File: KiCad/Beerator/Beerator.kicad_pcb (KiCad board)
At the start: 4 copper layers, 112 x 52 mm, 55 parts, among them SW1 SW_DPDT_x2, Y401 16MHz

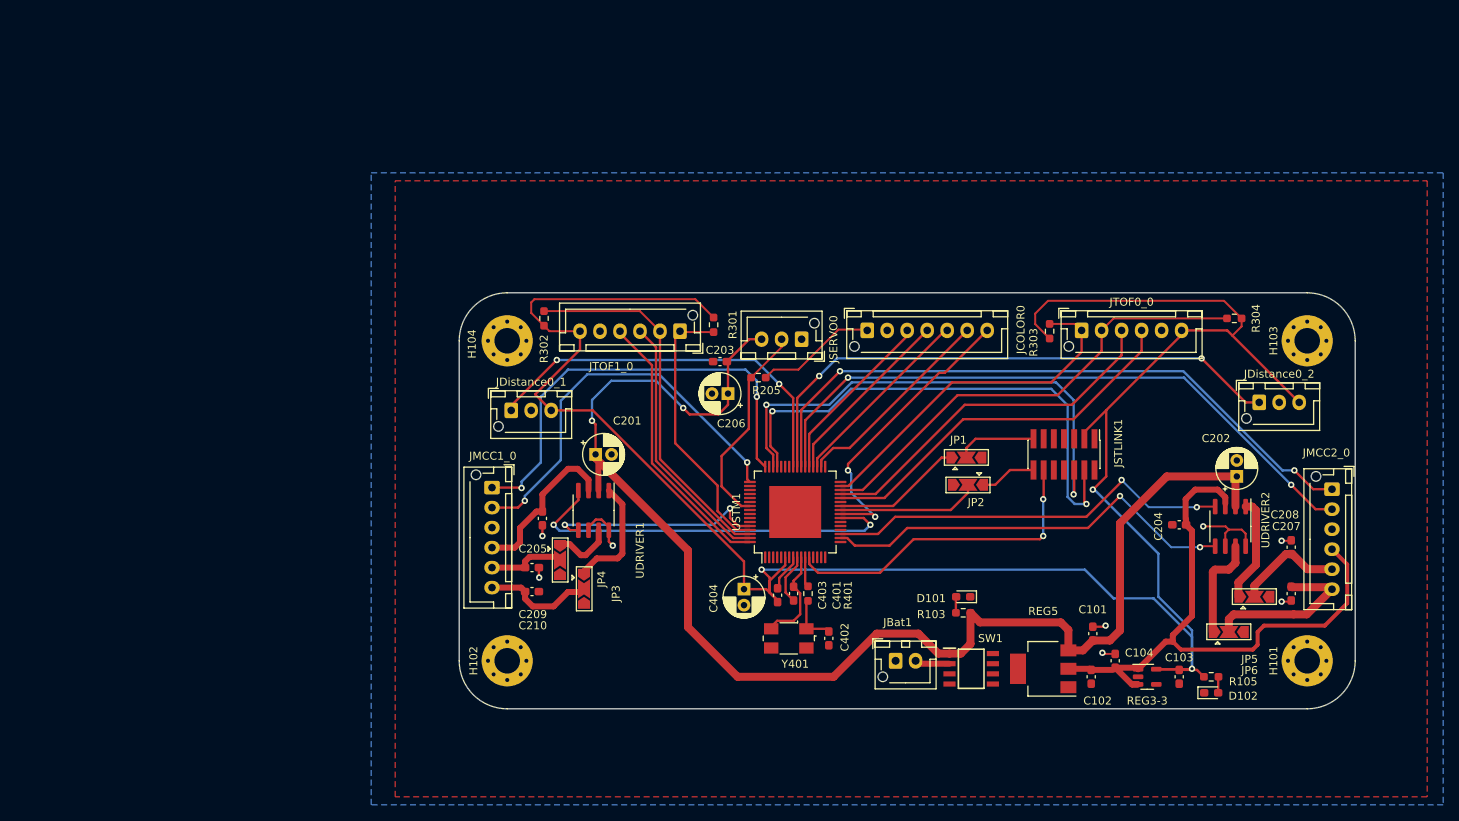
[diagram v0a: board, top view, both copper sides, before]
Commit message: pcb_v2
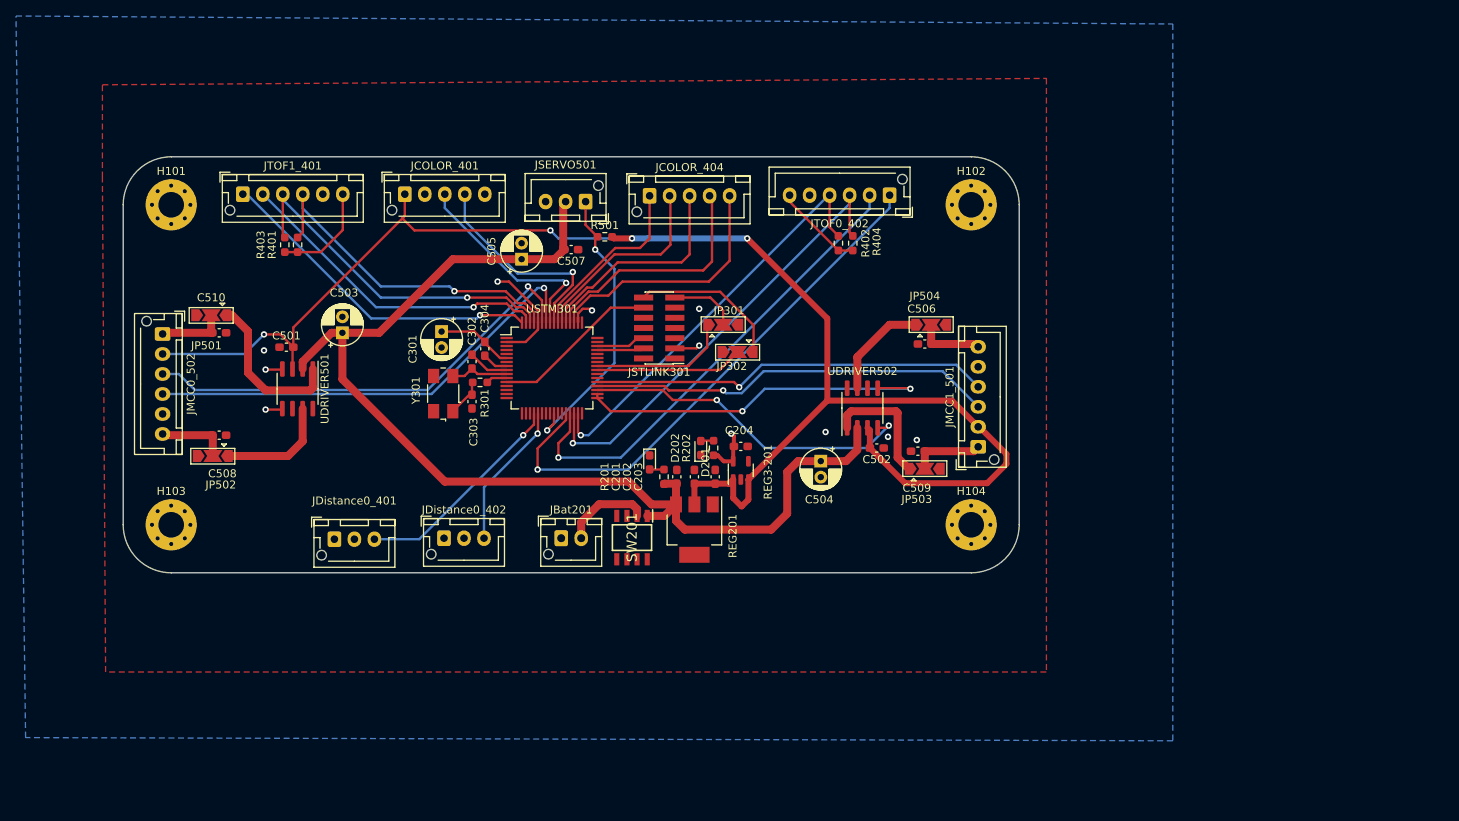
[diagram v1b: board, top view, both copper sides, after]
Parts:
- removed C101: 10uF, Capacitor_SMD:C_0603_1608Metric_Pad1.08x0.95mm_HandSolder
- removed C102: 22uF, Capacitor_SMD:C_0603_1608Metric_Pad1.08x0.95mm_HandSolder
- removed C103, C104: 1uF, Capacitor_SMD:C_0603_1608Metric_Pad1.08x0.95mm_HandSolder
- removed C205: 1µF, Capacitor_SMD:C_0603_1608Metric_Pad1.08x0.95mm_HandSolder
- removed C206: 100uF, Capacitor_THT:CP_Radial_D5.0mm_P2.00mm
- removed C207, C208, C209, C210: 0.1uF, Capacitor_SMD:C_0603_1608Metric_Pad1.08x0.95mm_HandSolder
- removed C401, C402: 15p, Capacitor_SMD:C_0603_1608Metric_Pad1.08x0.95mm_HandSolder
- removed C403: 100n, Capacitor_SMD:C_0603_1608Metric_Pad1.08x0.95mm_HandSolder
- removed C404: 4,7u, Capacitor_THT:CP_Radial_D5.0mm_P2.00mm
- removed D101, D102: LED_Small, LED_SMD:LED_0603_1608Metric_Pad1.05x0.95mm_HandSolder
- removed JBat1: Conn_01x02_Female, Connector_JST:JST_XH_B2B-XH-AM_1x02_P2.50mm_Vertical
- removed JCOLOR0: Conn_01x07_Female, Connector_JST:JST_XH_B7B-XH-AM_1x07_P2.50mm_Vertical
- removed JDistance0_1, JDistance0_2, JSERVO0: Conn_01x03_Female, Connector_JST:JST_XH_B3B-XH-AM_1x03_P2.50mm_Vertical
- removed JMCC1_0, JMCC2_0, JTOF0_0, JTOF1_0: Conn_01x06_Female, Connector_JST:JST_XH_B6B-XH-AM_1x06_P2.50mm_Vertical
- removed JP1, JP2, JP3, JP4, JP5, JP6: SolderJumper_2_Open, Jumper:SolderJumper-3_P2.0mm_Open_TrianglePad1.0x1.5mm
- removed JSTLINK1: Conn_02x07_Odd_Even, Connector_PinHeader_1.27mm:PinHeader_2x07_P1.27mm_Vertical_SMD
- removed R103, R105: 215, Resistor_SMD:R_0603_1608Metric_Pad0.98x0.95mm_HandSolder
- removed R205: 10k, Resistor_SMD:R_0603_1608Metric_Pad0.98x0.95mm_HandSolder
- removed R302, R303, R304: 1k, Resistor_SMD:R_0603_1608Metric_Pad0.98x0.95mm_HandSolder
- removed REG3-3: MCP1802x-xx02xOT, Package_TO_SOT_SMD:SOT-23-5
- removed REG5: AZ1117-5.0, Package_TO_SOT_SMD:SOT-223
- removed SW1: SW_DPDT_x2, SamacSys_Parts:NE555DR
- removed UDRIVER1, UDRIVER2: ZXBM5210-S, Package_SO:SOIC-8_3.9x4.9mm_P1.27mm
- removed USTM1: STM32G070RBT6, Package_QFP:LQFP-64-1EP_10x10mm_P0.5mm_EP6.5x6.5mm
- removed Y401: 16MHz, Crystal:Crystal_SMD_0603-4Pin_6.0x3.5mm
- added C301: 4,7u, Capacitor_THT:CP_Radial_D5.0mm_P2.00mm, F.Cu at (83.8, 65.8)
- added C302: 15p, Capacitor_SMD:C_0603_1608Metric_Pad1.08x0.95mm_HandSolder, F.Cu at (87.6, 69.6)
- added C303: 15p, Capacitor_SMD:C_0603_1608Metric_Pad1.08x0.95mm_HandSolder, F.Cu at (87.6, 74.6)
- added C304: 100n, Capacitor_SMD:C_0603_1608Metric_Pad1.08x0.95mm_HandSolder, F.Cu at (89.2, 68.0)
- added C501: 1µF, Capacitor_SMD:C_0603_1608Metric_Pad1.08x0.95mm_HandSolder, F.Cu at (64.4, 67.8)
- added C502: 1µF, Capacitor_SMD:C_0603_1608Metric_Pad1.08x0.95mm_HandSolder, F.Cu at (138.2, 80.4)
- added C503: 10µF, Capacitor_THT:CP_Radial_D5.0mm_P2.00mm, F.Cu at (71.4, 66.0)
- added C504: 10µF, Capacitor_THT:CP_Radial_D5.0mm_P2.00mm, F.Cu at (131.2, 82.0)
- added C505: 100uF, Capacitor_THT:CP_Radial_D5.0mm_P2.00mm, F.Cu at (93.8, 56.8)
- added C506: 0.1uF, Capacitor_SMD:C_0603_1608Metric_Pad1.08x0.95mm_HandSolder, F.Cu at (144.2, 67.4)
- added C507: 0.1uF, Capacitor_SMD:C_0603_1608Metric_Pad1.08x0.95mm_HandSolder, F.Cu at (100.0, 55.6)
- added C508: 0.1uF, Capacitor_SMD:C_0603_1608Metric_Pad1.08x0.95mm_HandSolder, F.Cu at (56.0, 78.8)
- added C509: 0.1uF, Capacitor_SMD:C_0603_1608Metric_Pad1.08x0.95mm_HandSolder, F.Cu at (143.3, 80.8)
- added C510: 0.1uF, Capacitor_SMD:C_0603_1608Metric_Pad1.08x0.95mm_HandSolder, F.Cu at (56.0, 66.0)
- added D201: LED_Small, LED_SMD:LED_0603_1608Metric_Pad1.05x0.95mm_HandSolder, F.Cu at (109.8, 82.2)
- added D202: LED_Small, LED_SMD:LED_0603_1608Metric_Pad1.05x0.95mm_HandSolder, F.Cu at (116.2, 80.4)
- added JBat201: Conn_01x02_Female, Connector_JST:JST_XH_B2B-XH-AM_1x02_P2.50mm_Vertical, F.Cu at (98.8, 91.7)
- added JCOLOR_401: Conn_01x05_Female, Connector_JST:JST_XH_B5B-XH-AM_1x05_P2.50mm_Vertical, F.Cu at (79.2, 48.7)
- added JCOLOR_404: Conn_01x05_Female, Connector_JST:JST_XH_B5B-XH-AM_1x05_P2.50mm_Vertical, F.Cu at (109.8, 48.9)
- added JDistance0_401: Conn_01x03_Female, Connector_JST:JST_XH_B3B-XH-AM_1x03_P2.50mm_Vertical, F.Cu at (70.4, 91.8)
- added JDistance0_402: Conn_01x03_Female, Connector_JST:JST_XH_B3B-XH-AM_1x03_P2.50mm_Vertical, F.Cu at (84.1, 91.7)
- added JMCC0_502: Conn_01x06_Female, Connector_JST:JST_XH_B6B-XH-AM_1x06_P2.50mm_Vertical, F.Cu at (48.9, 66.2)
- added JMCC1_501: Conn_01x06_Female, Connector_JST:JST_XH_B6B-XH-AM_1x06_P2.50mm_Vertical, F.Cu at (150.9, 80.2)
- added JP301: SolderJumper_2_Open, Jumper:SolderJumper-3_P2.0mm_Open_TrianglePad1.0x1.5mm, F.Cu at (119.0, 65.0)
- added JP302: SolderJumper_2_Open, Jumper:SolderJumper-3_P2.0mm_Open_TrianglePad1.0x1.5mm, F.Cu at (120.8, 68.4)
- added JP501: SolderJumper_2_Open, Jumper:SolderJumper-3_P2.0mm_Open_TrianglePad1.0x1.5mm, F.Cu at (55.0, 63.8)
- added JP502: SolderJumper_2_Open, Jumper:SolderJumper-3_P2.0mm_Open_TrianglePad1.0x1.5mm, F.Cu at (55.2, 81.4)
- added JP503: SolderJumper_2_Open, Jumper:SolderJumper-3_P2.0mm_Open_TrianglePad1.0x1.5mm, F.Cu at (144.2, 83.0)
- added JP504: SolderJumper_2_Open, Jumper:SolderJumper-3_P2.0mm_Open_TrianglePad1.0x1.5mm, F.Cu at (145.0, 65.0)
- added JSERVO501: Conn_01x03_Female, Connector_JST:JST_XH_B3B-XH-AM_1x03_P2.50mm_Vertical, F.Cu at (101.8, 49.6)
- added JSTLINK301: Conn_02x07_Odd_Even, Connector_PinHeader_1.27mm:PinHeader_2x07_P1.27mm_Vertical_SMD, F.Cu at (111.0, 65.4)
- added JTOF0_402: Conn_01x06_Female, Connector_JST:JST_XH_B6B-XH-AM_1x06_P2.50mm_Vertical, F.Cu at (139.8, 48.8)
- added JTOF1_401: Conn_01x06_Female, Connector_JST:JST_XH_B6B-XH-AM_1x06_P2.50mm_Vertical, F.Cu at (59.0, 48.7)
- added R201: 4,2k, Resistor_SMD:R_0603_1608Metric_Pad0.98x0.95mm_HandSolder, F.Cu at (111.6, 84.0)
- added R202: 300, Resistor_SMD:R_0603_1608Metric_Pad0.98x0.95mm_HandSolder, F.Cu at (117.8, 80.4)
- added R402: 1k, Resistor_SMD:R_0603_1608Metric_Pad0.98x0.95mm_HandSolder, F.Cu at (133.4, 54.8)
- added R403: 1k, Resistor_SMD:R_0603_1608Metric_Pad0.98x0.95mm_HandSolder, F.Cu at (64.2, 55.0)
- added R404: 1k, Resistor_SMD:R_0603_1608Metric_Pad0.98x0.95mm_HandSolder, F.Cu at (135.2, 54.8)
- added R501: 10k, Resistor_SMD:R_0603_1608Metric_Pad0.98x0.95mm_HandSolder, F.Cu at (104.2, 54.0)
- added REG201: AZ1117-5.0, Package_TO_SOT_SMD:SOT-223, F.Cu at (115.4, 90.6)
- added REG3-201: MCP1802x-xx02xOT, Package_TO_SOT_SMD:SOT-23-5, F.Cu at (121.2, 83.2)
- added SW201: SW_DPDT_x2, SamacSys_Parts:NE555DR, F.Cu at (107.6, 91.6)
- added UDRIVER501: ZXBM5210-S, Package_SO:SOIC-8_3.9x4.9mm_P1.27mm, F.Cu at (65.8, 73.0)
- added UDRIVER502: ZXBM5210-S, Package_SO:SOIC-8_3.9x4.9mm_P1.27mm, F.Cu at (136.4, 75.4)
- added USTM301: STM32G070RBT6, Package_QFP:LQFP-64_10x10mm_P0.5mm, F.Cu at (97.6, 70.4)
- added Y301: 16MHz, Crystal:Crystal_SMD_0603-4Pin_6.0x3.5mm, F.Cu at (84.0, 73.6)
- C201: value 10µF -> 10uF; footprint Capacitor_THT:CP_Radial_D5.0mm_P2.00mm -> Capacitor_SMD:C_0603_1608Metric_Pad1.08x0.95mm_HandSolder
- C202: value 10µF -> 22uF; footprint Capacitor_THT:CP_Radial_D5.0mm_P2.00mm -> Capacitor_SMD:C_0603_1608Metric_Pad1.08x0.95mm_HandSolder
- C203: value 0.1uF -> 1uF
- C204: value 1µF -> 1uF
- R301: value 1k -> 80
- R401: value 80 -> 1k
- moved H101 153.0 mm to (50.0, 50.0), turned to 0 degrees
- moved H103 143.9 mm to (50.0, 90.0), turned to 0 degrees
- moved H102 81.3 mm to (150.0, 50.0), turned to 0 degrees
- moved R401 77.3 mm to (65.8, 55.0)
- moved C202 67.8 mm to (115.4, 84.0)
- moved H104 62.4 mm to (150.0, 90.0), turned to 0 degrees
- moved C204 55.7 mm to (121.2, 80.2)
- moved R301 30.1 mm to (88.6, 72.2), turned to 0 degrees
- moved C203 14.4 mm to (118.0, 84.0), turned to 90 degrees
- moved C201 10.5 mm to (113.2, 84.0), turned to 90 degrees
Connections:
- C201 pad 1: 7.2 -> +BATT
- C202 pad 1: 7.2 -> +5V
- C203 pad 1: GND -> +5V
- C203 pad 2: 7.2 -> GND
- C204 pad 1: GND -> +3.3V
- C204 pad 2: 5 -> GND
- R301 pad 1: TOF2_SDA -> Net-(C303-Pad2)
- R301 pad 2: 3.3 -> Net-(R301-Pad2)
- R401 pad 1: Net-(C402-Pad2) -> +3.3V
- R401 pad 2: Net-(R401-Pad2) -> TOF2_SDA
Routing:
- net 3.3: track 277.2 -> 0.00 mm, vias 3 -> 0
- net +5V: track 0.00 -> 196.9 mm, vias 0 -> 4
- net 7.2: track 172.2 -> 0.00 mm, vias 2 -> 0
- net +BATT: track 0.00 -> 143.5 mm
- net 5: track 114.0 -> 0.00 mm
- net SWDIO: track 64.8 -> 5.87 mm, vias 2 -> 0
- net SWCLK: track 63.4 -> 6.19 mm, vias 2 -> 0
- net IR2-OUT: track 70.7 -> 27.3 mm, vias 2 -> 1
- net +3.3V: track 0.00 -> 43.3 mm, vias 0 -> 2
- net PHASE_A_M2: track 81.6 -> 50.2 mm, vias 2 -> 1
- net IR1-OUT: track 48.8 -> 18.4 mm, vias 2 -> 1
- net PHASE_B_M2: track 80.7 -> 51.6 mm, vias 2 -> 1
- net NPWM_D1: track 27.6 -> 55.1 mm
- net TCS-LED: track 0.00 -> 27.0 mm, vias 0 -> 1
- net TCS-OE: track 0.00 -> 26.6 mm, vias 0 -> 1
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- added copper zone on In2.Cu, net +3.3V
- removed copper zone on In2.Cu, net 5
